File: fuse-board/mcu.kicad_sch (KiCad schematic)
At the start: 65 parts, among them IC1 TMUX1308QPWRQ1, J1 FTSH-107-01-F-DV-K-P-TR, J10 Conn_01x03, J11 Conn_01x03, J12 Conn_01x03, J13 Conn_01x03, J14 Conn_01x03, J6 Conn_01x03, J7 Conn_01x03, J8 Conn_01x03, J9 Conn_01x03, SW1 Y97KT23B5NAFP, U1 STM32G491KCUx, U13 74AHCT1G125, Y1 ECS-240-8-37B-CKY-TR

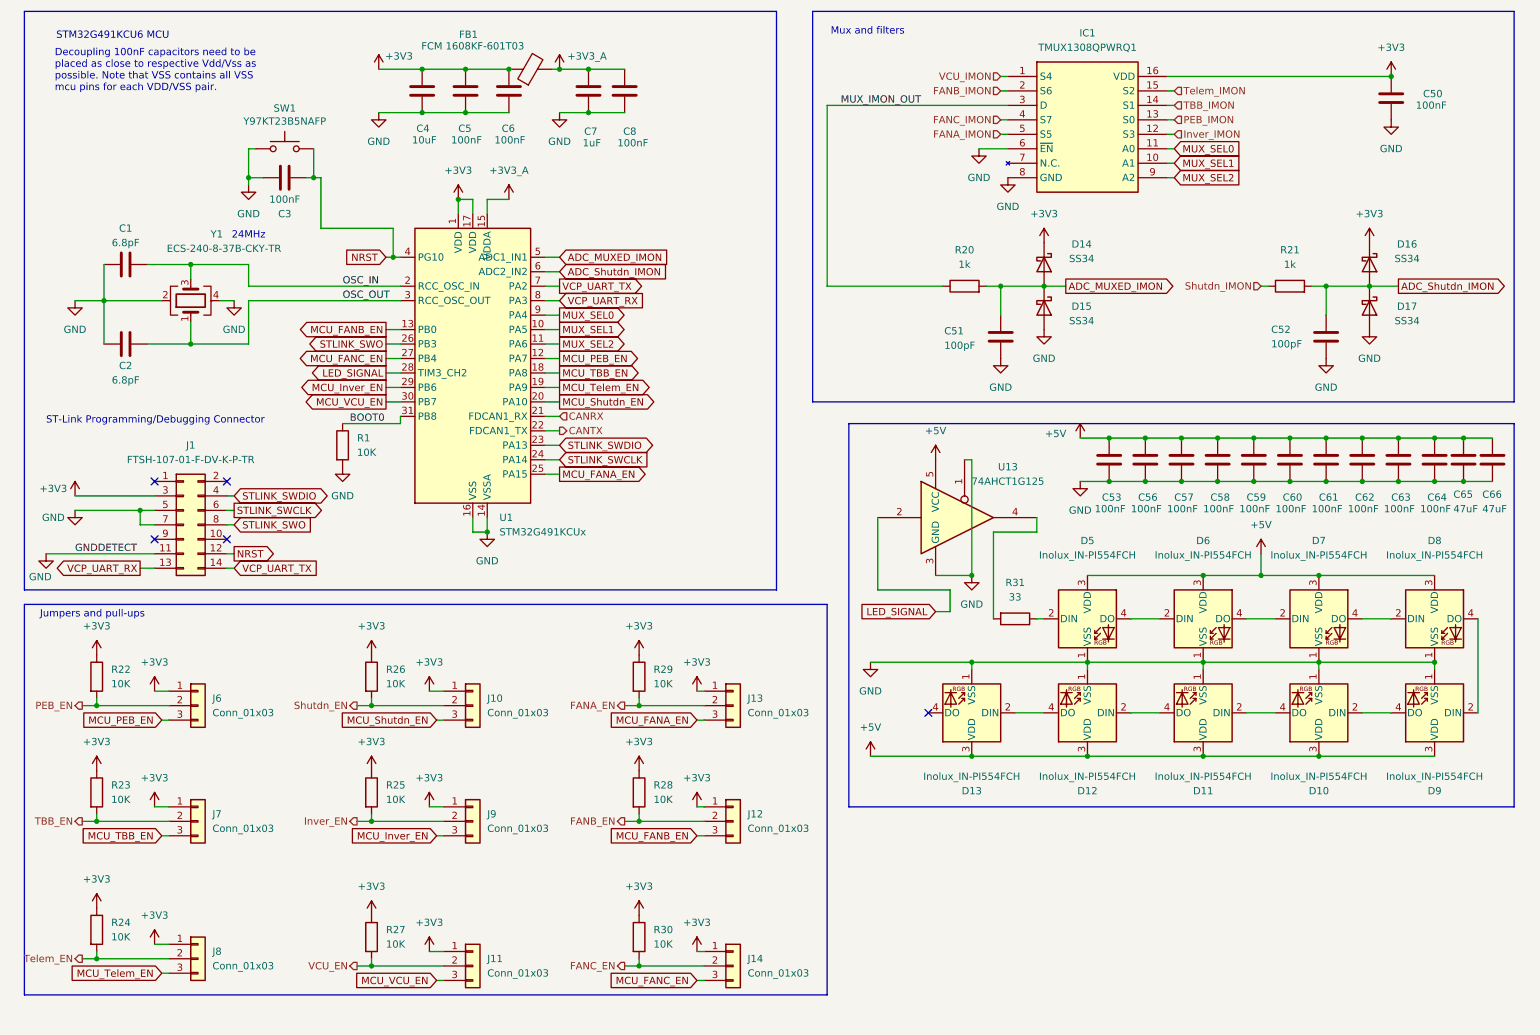
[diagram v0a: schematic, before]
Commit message: mcu -> g441, remove jumpers
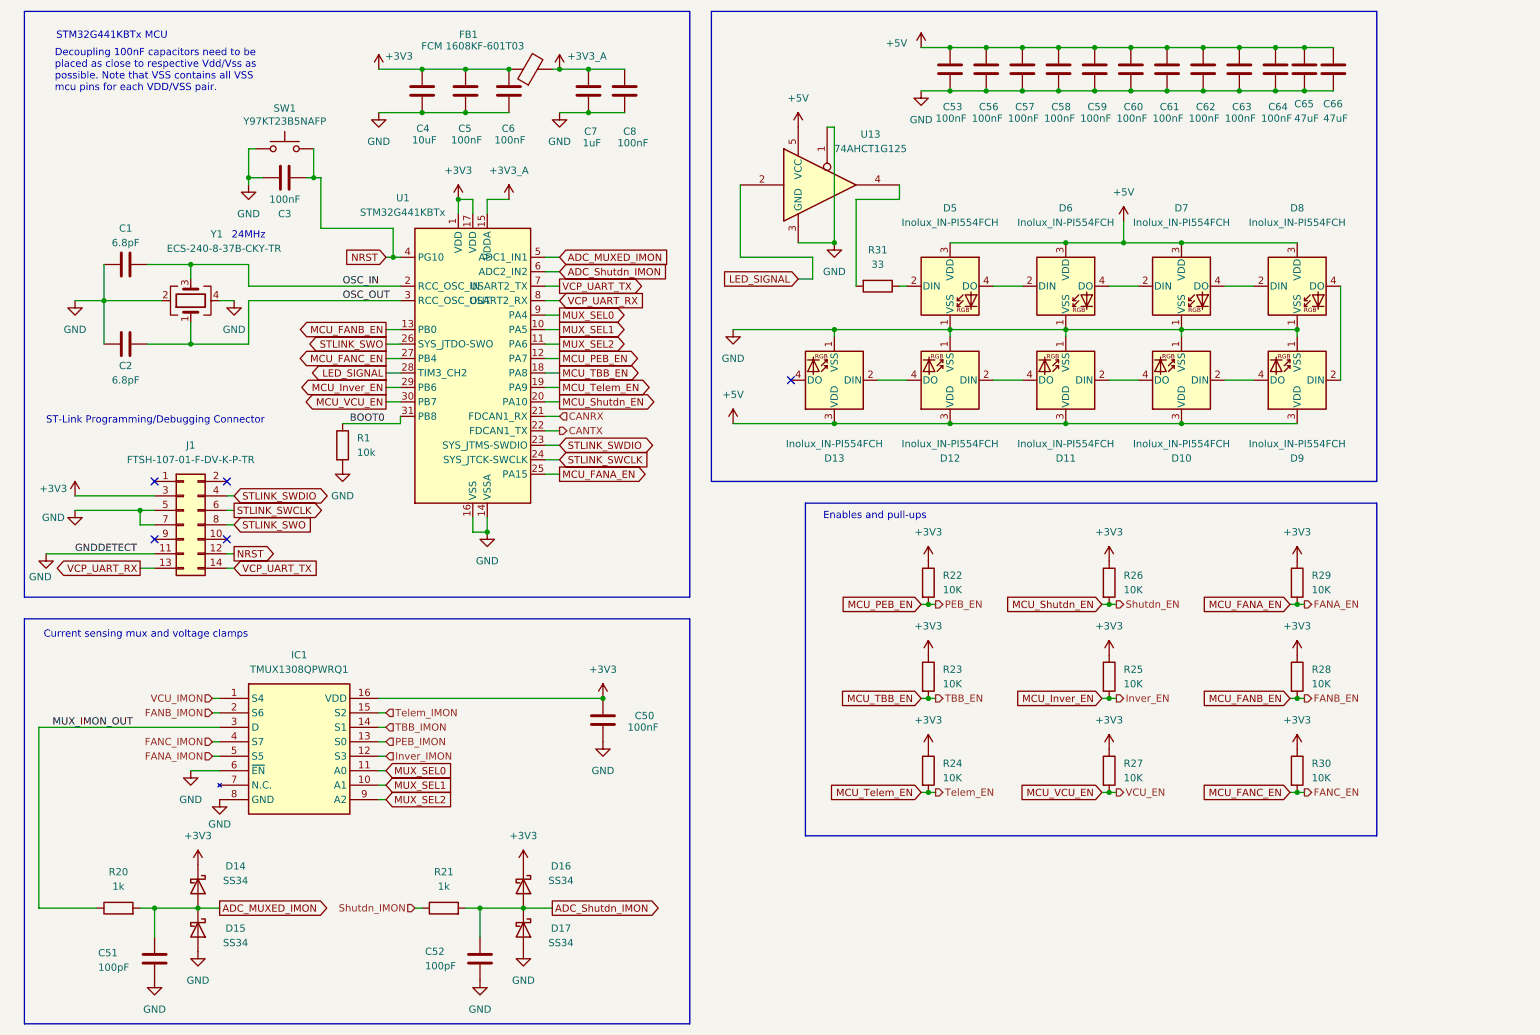
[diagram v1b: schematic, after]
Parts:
- removed J10, J11, J12, J13, J14, J6, J7, J8, J9: Conn_01x03, Connector_PinHeader_2.54mm:PinHeader_1x03_P2.54mm_Vertical, symbol Connector_Generic:Conn_01x03
- removed U1: STM32G491KCUx, Package_DFN_QFN:QFN-32-1EP_5x5mm_P0.5mm_EP3.45x3.45mm, symbol MCU_ST_STM32G4:STM32G491KCUx
- added U1: STM32G441KBTx, Package_QFP:LQFP-32_7x7mm_P0.8mm, symbol MCU_ST_STM32G4:STM32G441KBTx
- C1, C2: Digi PN (none) -> 311-3874-1-ND; Digi URL (none) -> https://www.digikey.com/en/products/detail/yageo/CC0603DRNP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; Digikey Part Number 311-3874-1-ND -> (none); Digikey URL https://www.digikey.com/en/products/detail/yageo/CC0603DRNP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 -> (none); MFG (none) -> Yageo; MFG PN (none) -> CC0603DRNPO9BN6R8; Manufacturer YAGEO -> (none); Manufacturer Part Number CC0603DRNPO9BN6R8 -> (none)
- C3, C5, C6, C8: Digi PN (none) -> 311-1344-1-ND; Digi URL (none) -> https://www.digikey.com/en/products/detail/yageo/CC0603KRX7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; Digikey Part Number 311-1344-1-ND -> (none); Digikey URL https://www.digikey.com/en/products/detail/yageo/CC0603KRX7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 -> (none); MFG (none) -> Yageo; MFG PN (none) -> CC0603KRX7R9BB104; Manufacturer YAGEO -> (none); Manufacturer Part Number CC0603KRX7R9BB104 -> (none)
- C4: Digi PN (none) -> 1276-CL10A106KO8NQNCCT-ND; Digi URL (none) -> https://www.digikey.com/en/products/detail/samsung-electro-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; Digikey Part Number 1276-CL10A106KO8NQNCCT-ND -> (none); Digikey URL https://www.digikey.com/en/products/detail/samsung-electro-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 -> (none); MFG (none) -> Samsung Electro-Mechanics; MFG PN (none) -> CL10A106KO8NQNC; Manufacturer Samsung Electro-Mechanics -> (none); Manufacturer Part Number CL10A106KO8NQNC -> (none)
- C7: Digi PN (none) -> 1276-CL10B105KB9VPJCCT-ND; Digi URL (none) -> https://www.digikey.com/en/products/detail/samsung-electro-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; Digikey Part Number 1276-CL10B105KB9VPJCCT-ND -> (none); Digikey URL https://www.digikey.com/en/products/detail/samsung-electro-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 -> (none); MFG (none) -> Samsung Electro-Mechanics; MFG PN (none) -> CL10B105KB9VPJC; Manufacturer Samsung Electro-Mechanics -> (none); Manufacturer Part Number CL10B105KB9VPJC -> (none)
- FB1: Digi PN (none) -> 4816-FCM1608KF-601T03CT-ND; Digi URL (none) -> https://www.digikey.com/en/products/detail/tai-tech-advance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; Digikey Part Number 4816-FCM1608KF-601T03CT-ND -> (none); Digikey URL https://www.digikey.com/en/products/detail/tai-tech-advance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 -> (none); MFG (none) -> TAI-TECH Advanced Electronics Co., Ltd.; MFG PN (none) -> FCM 1608KF-601T03; Manufacturer TAI-TECH Advanced Electronics Co., Ltd. -> (none); Manufacturer Part Number FCM 1608KF-601T03 -> (none)
- J1: Digi PN (none) -> SAM13170CT-ND; Digi URL (none) -> https://www.digikey.com/en/products/detail/samtec-inc/FTSH-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; Digikey Part Number SAM13170CT-ND -> (none); Digikey URL https://www.digikey.com/en/products/detail/samtec-inc/FTSH-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 -> (none); MFG (none) -> Samtec Inc.; MFG PN (none) -> FTSH-107-01-F-DV-K-P-TR; Manufacturer Samtec Inc. -> (none); Manufacturer Part Number FTSH-107-01-F-DV-K-P-TR -> (none)
- R1: value 10K -> 10k; Digi PN (none) -> 311-10KLDCT-ND; Digi URL (none) -> https://www.digikey.com/en/products/detail/yageo/AC0603FR-0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; Digikey Part Number 311-10KLDCT-ND -> (none); Digikey URL https://www.digikey.com/en/products/detail/yageo/AC0603FR-0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 -> (none); MFG (none) -> Yageo; MFG PN (none) -> AC0603FR-0710KL; Manufacturer YAGEO -> (none); Manufacturer Part Number AC0603FR-0710KL -> (none)
- SW1: Digi PN (none) -> 108-Y97KT23B5NAFPCT-ND; Digi URL (none) -> https://www.digikey.com/en/products/detail/c-k/y97kt23b5naf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; Digikey Part Number 108-Y97KT23B5NAFPCT-ND -> (none); Digikey URL https://www.digikey.com/en/products/detail/c-k/y97kt23b5naf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 -> (none); MFG (none) -> C&K; MFG PN (none) -> Y97KT23B5NAFP; Manufacturer C&K -> (none); Manufacturer Part Number Y97KT23B5NAFPY97KT23B5NAFP -> (none)
- Y1: Digi PN (none) -> XC3063CT-ND; Digi URL (none) -> https://www.digikey.com/en/products/detail/ecs-inc/ECS-240-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; Digikey Part Number XC3063CT-ND -> (none); Digikey URL https://www.digikey.com/en/products/detail/ecs-inc/ECS-240-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 -> (none); MFG (none) -> ECS; MFG PN (none) -> ECS-240-8-37B-CKY-TR; Manufacturer ECS -> (none); Manufacturer Part Number ECS-240-8-37B-CKY-TR -> (none)
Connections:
- net FANA_EN is gone; now on net MCU_FANA_EN: R29.2
- net FANB_EN is gone; now on net MCU_FANB_EN: R28.2
- net FANC_EN is gone; now on net MCU_FANC_EN: R30.2
- net Inver_EN is gone; now on net MCU_Inver_EN: R25.2
- net PEB_EN is gone; now on net MCU_PEB_EN: R22.2
- net Shutdn_EN is gone; now on net MCU_Shutdn_EN: R26.2
- net TBB_EN is gone; now on net MCU_TBB_EN: R23.2
- net Telem_EN is gone; now on net MCU_Telem_EN: R24.2
- net VCU_EN is gone; now on net MCU_VCU_EN: R27.2
- net +3V3: now also U1.1 (VDD), U1.17 (VDD)
- net +3V3_A: now also U1.15 (VDDA)
- net ADC_MUXED_IMON: now also U1.5 (PA0)
- net ADC_Shutdn_IMON: now also U1.6 (PA1)
- net BOOT0: now also U1.31 (PB8)
- net CANRX: now also U1.21 (PA11)
- net CANTX: now also U1.22 (PA12)
- net GND: now also U1.14 (VSSA), U1.16 (VSS), U1.32 (VSS)
- net LED_SIGNAL: now also U1.28 (PB5)
- net MCU_FANA_EN: now also U1.25 (PA15)
- net MCU_FANB_EN: now also U1.13 (PB0)
- net MCU_FANC_EN: now also U1.27 (PB4)
- net MCU_Inver_EN: now also U1.29 (PB6)
- net MCU_PEB_EN: now also U1.12 (PA7)
- net MCU_Shutdn_EN: now also U1.20 (PA10)
- net MCU_TBB_EN: now also U1.18 (PA8)
- net MCU_Telem_EN: now also U1.19 (PA9)
- net MCU_VCU_EN: now also U1.30 (PB7)
- net MUX_SEL0: now also U1.9 (PA4)
- net MUX_SEL1: now also U1.10 (PA5)
- net MUX_SEL2: now also U1.11 (PA6)
- net NRST: now also U1.4 (PG10)
- net OSC_IN: now also U1.2 (PF0)
- net OSC_OUT: now also U1.3 (PF1)
- net STLINK_SWCLK: now also U1.24 (PA14)
- net STLINK_SWDIO: now also U1.23 (PA13)
- net STLINK_SWO: now also U1.26 (PB3)
- net VCP_UART_RX: now also U1.8 (PA3)
- net VCP_UART_TX: now also U1.7 (PA2)
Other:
- note added: "Current sensing mux and voltage clamps"
- note added: "Enables and pull-ups"
- note added: "STM32G441KBTx MCU"
- note removed: "Jumpers and pull-ups"
- note removed: "Mux and filters"
- note removed: "STM32G491KCU6 MCU"
- moved on the sheet: C53, C56, C57, C58, C59, C60, C61, C62, C63, C64, C65, C66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
